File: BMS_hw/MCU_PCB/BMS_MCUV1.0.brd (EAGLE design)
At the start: 60 x 30 mm, 51 parts, among them IC2 SST25VF020B804ISA, J1 22-27-2051-05, J2 22-27-2051-05, J3 22-27-2041-04, J4 22-27-2051-05, U1 NCP1117LP-PG, U2 NCP1117LP-PG

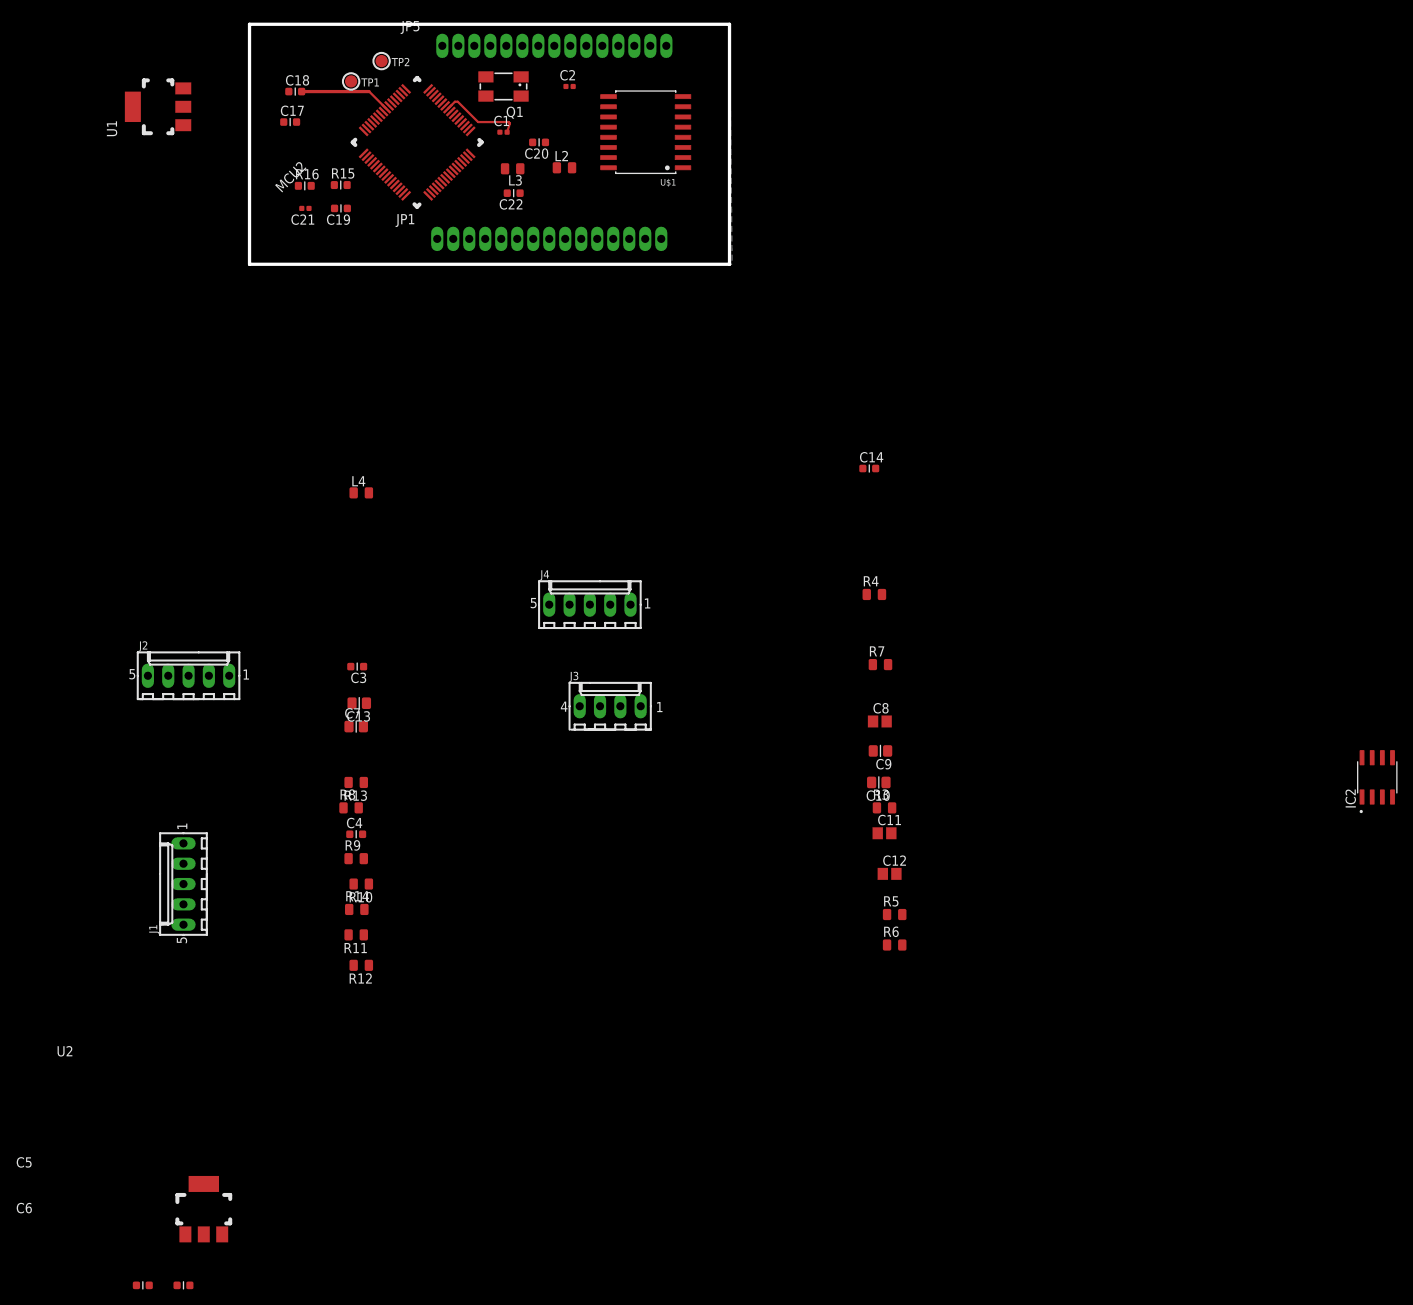
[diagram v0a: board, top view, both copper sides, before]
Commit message: brd layout and sch updated!
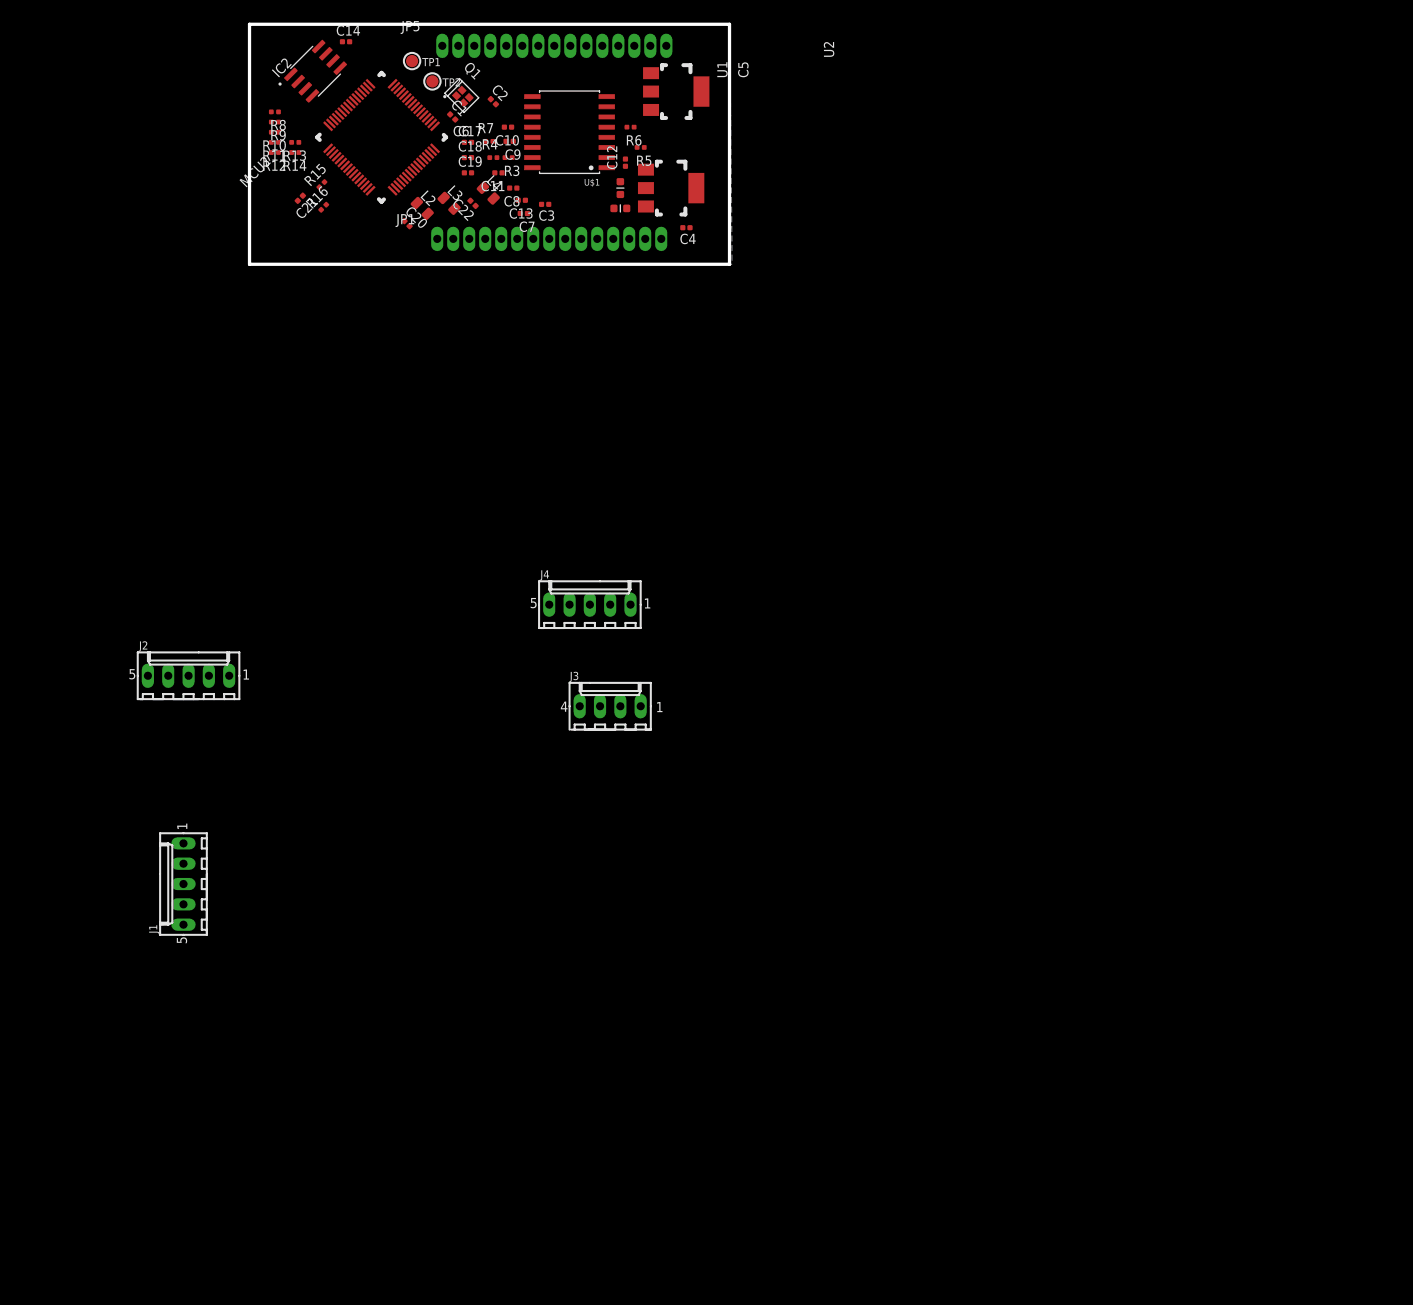
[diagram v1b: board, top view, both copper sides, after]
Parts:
- C10, C13, C7, C9: device ipc-7351-capacitor:CAPC2012X145AN -> ipc-7351-capacitor:CAPC1005X60N
- C11, C12, C8: device adafruit:C0805 -> ipc-7351-capacitor:CAPC1005X60N
- C14, C17, C18, C19, C20, C22, C3, C4: device ipc-7351-capacitor:CAPC1608X92N -> ipc-7351-capacitor:CAPC1005X60N
- Q1: value (none) -> CRYSTALS-GND-LID-IQXC-42; device adafruit:CTS406 -> IQD-Frequency-Products:2.0X1.6-4-PAD
- R10, R11, R12, R13, R14, R3, R4, R5, R6, R7, R8, R9: device ipc-7351-resistor:RESC2012X70N -> ipc-7351-resistor:RESC1005X40AN
- R15, R16: device ipc-7351-resistor:RESC1608X55N -> ipc-7351-resistor:RESC1005X40AN
- moved IC2 159.4 mm to (8.26, 24.1), turned to 45 degrees
- moved C5 149.6 mm to (46.4, 9.53), turned to 270 degrees
- moved C6 145.3 mm to (46.4, 6.99)
- moved U2 140.4 mm to (52.7, 9.53), turned to 270 degrees
- moved R6 107.4 mm to (47.6, 17.1), turned to 180 degrees
- moved R12 102.2 mm to (3.17, 14.0)
- moved R5 101.0 mm to (48.9, 14.6), turned to 180 degrees
- moved R11 99.6 mm to (3.17, 15.2)
- moved C11 95.6 mm to (31.1, 11.4), turned to 180 degrees
- moved R14 94.9 mm to (5.71, 14.0), turned to 180 degrees
- moved C12 94.8 mm to (47.0, 12.7), turned to 90 degrees
- moved R10 94.6 mm to (3.17, 16.5)
- moved C10 94.1 mm to (32.3, 17.1)
- moved R3 93.9 mm to (32.4, 13.3), turned to 180 degrees
- moved R9 92.6 mm to (3.17, 17.8), turned to 180 degrees
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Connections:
- new net N$3: C12.1, U$1.1
- net 3.3V: no longer C12.1, U$1.1
- net GND: now also Q1.2, Q1.4
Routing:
- net GND: track 21.9 -> 0.00 mm
